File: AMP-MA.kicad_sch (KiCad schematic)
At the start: 54 parts, among them Q1 2N5484, Q12 2N5484, Q13 2N5484, Q2 2N5484, U2 LM1875, U3 TL072

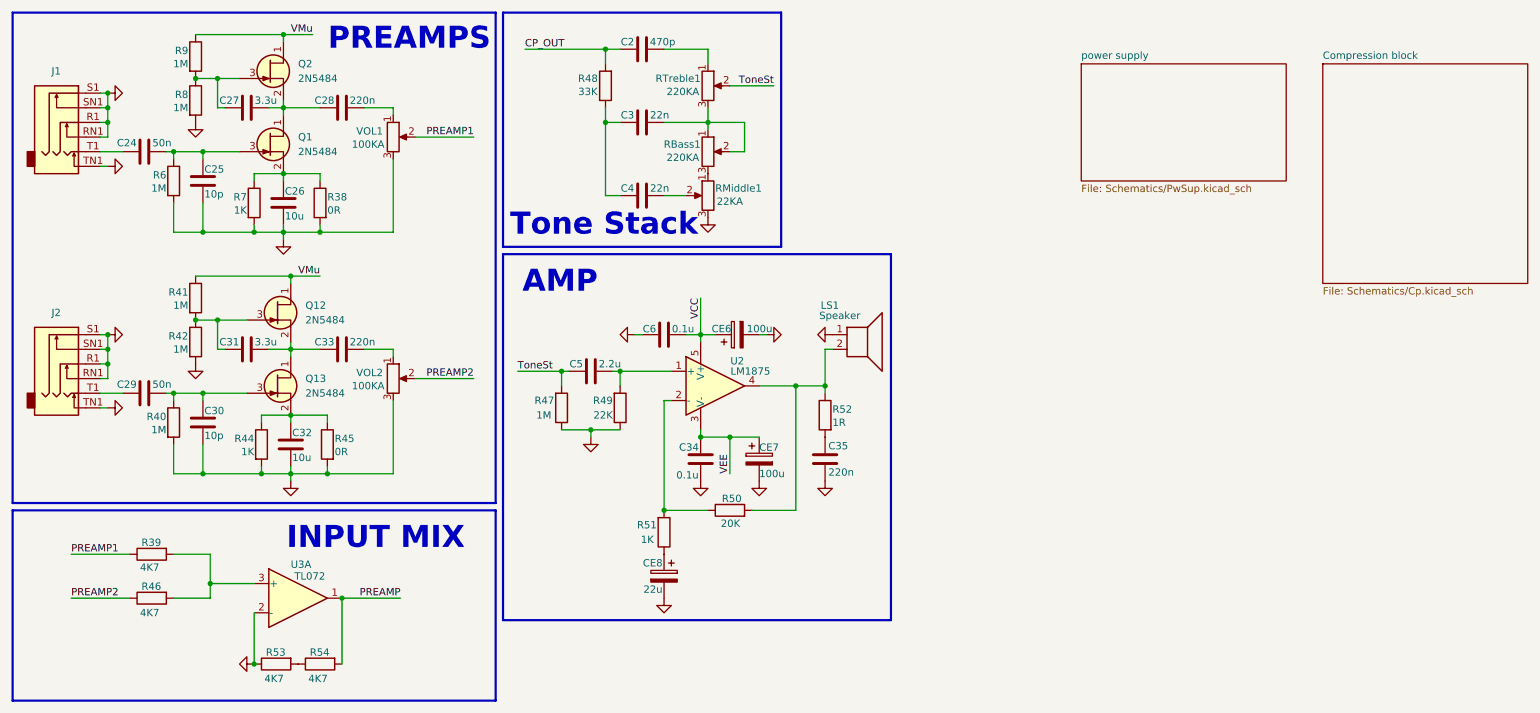
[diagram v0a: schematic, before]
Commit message: Schem upd & added .gitignore
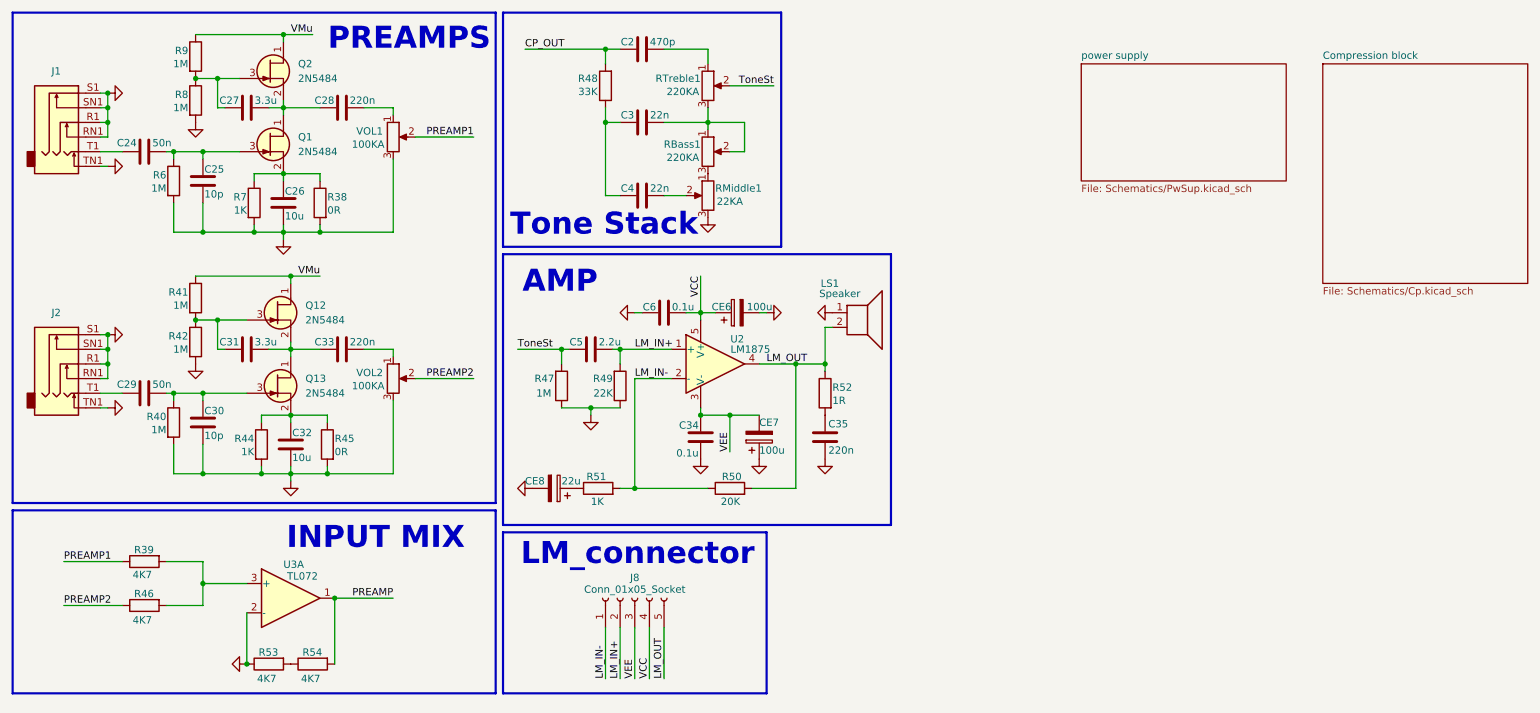
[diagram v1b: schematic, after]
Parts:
- added J8: Conn_01x05_Socket, symbol Connector:Conn_01x05_Socket
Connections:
- net GND: now also CE7.1; no longer CE7.2
- net VCC: now also J8.4 (Pin_4)
- net VEE: now also CE7.2, J8.3 (Pin_3); no longer CE7.1
- net LM_OUT: now reaches LS1.2, R50.2, R52.1, U2.4
- net LM_OUT: now also J8.5 (Pin_5)
- net LM_IN-: now reaches R50.1, R51.2, U2.2 (-)
- net LM_IN-: now also J8.1 (Pin_1)
- net LM_IN+: now reaches C5.2, R49.2, U2.1 (+)
- net LM_IN+: now also J8.2 (Pin_2)
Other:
- note added: "LM_connector"
- moved on the sheet: C34, C35, C5, C6, CE6, CE7, CE8, LS1, R39, R46, R47, R49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
